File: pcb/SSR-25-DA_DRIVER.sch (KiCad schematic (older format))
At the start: 3 parts, among them Q3 SS9013_J3

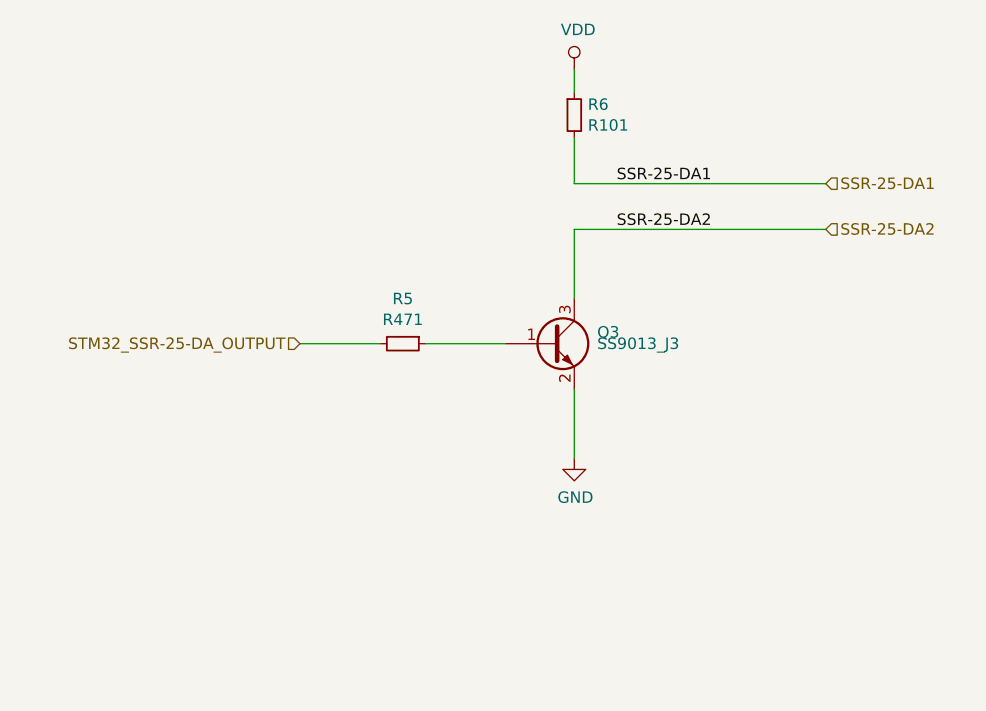
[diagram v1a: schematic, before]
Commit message: update,
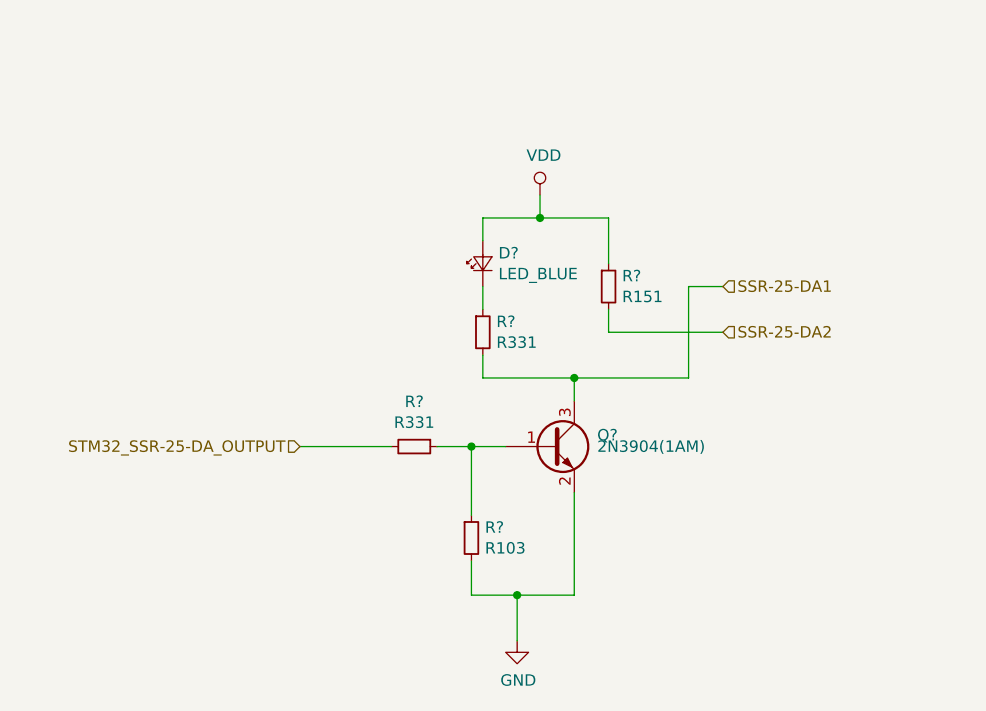
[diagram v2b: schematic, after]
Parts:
- removed Q3: SS9013_J3, Package_TO_SOT_SMD:SOT-23_Handsoldering, symbol taobao-transistor:SS9013_J3
- removed R5: R471, Resistor_SMD:R_0805_2012Metric_Pad1.15x1.40mm_HandSolder, symbol taobao-r:R471
- removed R6: R101, Resistor_SMD:R_0805_2012Metric_Pad1.15x1.40mm_HandSolder, symbol taobao-r:R101
- added D?: LED_BLUE, LED_SMD:LED_0805_2012Metric_Pad1.15x1.40mm_HandSolder, symbol taobao-components:LED_RED
- added Q?: 2N3904(1AM), Package_TO_SOT_SMD:SOT-23_Handsoldering, symbol taobao-transistor:2N3904(1AM)
- added R? (x2): R331, Resistor_SMD:R_0805_2012Metric_Pad1.15x1.40mm_HandSolder, symbol taobao-r:R331
- added R?: R103, Resistor_SMD:R_0805_2012Metric_Pad1.15x1.40mm_HandSolder, symbol taobao-r:R103
- added R?: R151, Resistor_SMD:R_0805_2012Metric_Pad1.15x1.40mm_HandSolder, symbol taobao-r:R151
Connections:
- net GND: now also Q?.2 (E), R?.2
- net SSR-25-DA1: now also Q?.3 (C), R?.2
- net SSR-25-DA2: now also R?.2
- net STM32_SSR-25-DA_OUTPUT: now also R?.2
- net VDD: now also D?.2 (A), R?.1
- new net: Q?.1 (B), R?.1, R?.1
- new net: D?.1 (K), R?.1
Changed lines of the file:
@@
 Comment4 ""
 $EndDescr
+Text HLabel 5050 3550 0    50   Input ~ 0
+STM32_SSR-25-DA_OUTPUT
 $Comp
-L power:VDD #PWR013
-U 1 1 5BCB697F
-P 6250 1900
-F 0 "#PWR013" H 6250 1750 50  0001 C CNN
-F 1 "VDD" H 6267 2073 50  0000 C CNN
-F 2 "" H 6250 1900 50  0001 C CNN
-F 3 "" H 6250 1900 50  0001 C CNN
-	1    6250 1900
-	1    0    0    -1
+L taobao-r:R331 R?
+U 1 1 5BDCB66A
+P 5550 3550
+AR Path="/5BCB4A39/5BDCB66A" Ref="R?"  Part="1"
+AR Path="/5BE41138/5BDCB66A" Ref="R?"  Part="1"
+AR Path="/5BCB679F/5BDCB66A" Ref="R?"  Part="1"
+F 0 "R?" V 5354 3550 50  0000 C CNN
+F 1 "R331" V 5445 3550 50  0000 C CNN
+F 2 "Resistor_SMD:R_0805_2012Metric_Pad1.15x1.40mm_HandSolder" H 5550 3550 50  0001 C CNN
+F 3 "~" H 5550 3550 50  0001 C CNN
+	1    5550 3550
+	0    1    1    0
 $EndComp
 $Comp
-L taobao-r:R101 R6
-U 1 1 5BCB69F8
-P 6250 2100
-F 0 "R6" H 6309 2146 50  0000 L CNN
-F 1 "R101" H 6309 2055 50  0000 L CNN
-F 2 "Resistor_SMD:R_0805_2012Metric_Pad1.15x1.40mm_HandSolder" H 6250 2100 50  0001 C CNN
-F 3 "~" H 6250 2100 50  0001 C CNN
-	1    6250 2100
-	1    0    0    -1
-$EndComp
-$Comp
-L taobao-r:R471 R5
-U 1 1 5BCB6A7C
-P 5500 3100
-F 0 "R5" V 5304 3100 50  0000 C CNN
-F 1 "R471" V 5395 3100 50  0000 C CNN
-F 2 "Resistor_SMD:R_0805_2012Metric_Pad1.15x1.40mm_HandSolder" H 5500 3100 50  0001 C CNN
-F 3 "~" H 5500 3100 50  0001 C CNN
-	1    5500 3100
-	0    1    1    0
-$EndComp
-Text Label 6850 2400 2    50   ~ 0
-SSR-25-DA1
-Text Label 6850 2600 2    50   ~ 0
-SSR-25-DA2
-Text HLabel 5050 3100 0    50   Input ~ 0
-STM32_SSR-25-DA_OUTPUT
-Wire Wire Line
-	5050 3100 5400 3100
-$Comp
-L power:GND #PWR014
-U 1 1 5BCB6BDC
-P 6250 3600
-F 0 "#PWR014" H 6250 3350 50  0001 C CNN
-F 1 "GND" H 6255 3427 50  0000 C CNN
-F 2 "" H 6250 3600 50  0001 C CNN
-F 3 "" H 6250 3600 50  0001 C CNN
-	1    6250 3600
+L taobao-r:R103 R?
+U 1 1 5BDCB672
+P 5800 3950
+AR Path="/5BCB4A39/5BDCB672" Ref="R?"  Part="1"
+AR Path="/5BE41138/5BDCB672" Ref="R?"  Part="1"
+AR Path="/5BCB679F/5BDCB672" Ref="R?"  Part="1"
+F 0 "R?" H 5859 3996 50  0000 L CNN
+F 1 "R103" H 5859 3905 50  0000 L CNN
+F 2 "Resistor_SMD:R_0805_2012Metric_Pad1.15x1.40mm_HandSolder" H 5800 3950 50  0001 C CNN
+F 3 "~" H 5800 3950 50  0001 C CNN
+	1    5800 3950
 	1    0    0    -1
 $EndComp
 Wire Wire Line
-	6250 3300 6250 3600
+	5050 3550 5450 3550
 Wire Wire Line
-	5600 3100 5950 3100
+	5650 3550 5800 3550
 Wire Wire Line
-	6250 2200 6250 2400
+	5800 3550 5800 3850
 Wire Wire Line
-	6250 1900 6250 2000
+	5950 3550 5800 3550
+Connection ~ 5800 3550
 Wire Wire Line
-	6250 2600 6250 2900
-Text HLabel 7350 2400 2    50   Input ~ 0
-SSR-25-DA1
-Text HLabel 7350 2600 2    50   Input ~ 0
-SSR-25-DA2
+	5800 4050 5800 4200
 Wire Wire Line
-	6250 2400 7350 2400
+	5800 4200 6000 4200
 Wire Wire Line
-	6250 2600 7350 2600
+	6250 4200 6250 3750
 $Comp
-L taobao-transistor:SS9013_J3 Q3
-U 1 1 5BCBD15E
-P 6150 3100
-AR Path="/5BCBD15E" Ref="Q3"  Part="1"
-AR Path="/5BCB679F/5BCBD15E" Ref="Q3"  Part="1"
-F 0 "Q3" H 6350 3150 50  0000 L CNN
-F 1 "SS9013_J3" H 6350 3100 50  0000 L CNN
-F 2 "Package_TO_SOT_SMD:SOT-23_Handsoldering" H 6350 3025 50  0001 L CIN
-F 3 "https://www.fairchildsemi.com/datasheets/2N/2N3904.pdf" H 6150 3100 50  0001 L CNN
-	1    6150 3100
+L power:GND #PWR?
+U 1 1 5BDCB681
+P 6000 4400
+AR Path="/5BCB4A39/5BDCB681" Ref="#PWR?"  Part="1"
+AR Path="/5BE41138/5BDCB681" Ref="#PWR?"  Part="1"
+F 0 "#PWR?" H 6000 4150 50  0001 C CNN
+F 1 "GND" H 6005 4227 50  0000 C CNN
+F 2 "" H 6000 4400 50  0001 C CNN
+F 3 "" H 6000 4400 50  0001 C CNN
+	1    6000 4400
 	1    0    0    -1
 $EndComp
+Wire Wire Line
+	6000 4400 6000 4200
+Connection ~ 6000 4200
+Wire Wire Line
+	6000 4200 6250 4200
+$Comp
+L taobao-components:LED_RED D?
+U 1 1 5BDCB68A
+P 5850 2750
+AR Path="/5BCB4A39/5BDCB68A" Ref="D?"  Part="1"
+AR Path="/5BE41138/5BDCB68A" Ref="D?"  Part="1"
+AR Path="/5BCB679F/5BDCB68A" Ref="D?"  Part="1"
+F 0 "D?" V 5896 2682 50  0000 R CNN
+F 1 "LED_BLUE" V 5805 2682 50  0000 R CNN
+F 2 "LED_SMD:LED_0805_2012Metric_Pad1.15x1.40mm_HandSolder" V 5850 2750 50  0001 C CNN
+F 3 "~" V 5850 2750 50  0001 C CNN
+	1    5850 2750
+	0    -1   -1   0
+$EndComp
+$Comp
+L taobao-r:R331 R?
+U 1 1 5BDCB691
+P 5850 3050
+AR Path="/5BCB4A39/5BDCB691" Ref="R?"  Part="1"
+AR Path="/5BE41138/5BDCB691" Ref="R?"  Part="1"
+AR Path="/5BCB679F/5BDCB691" Ref="R?"  Part="1"
+F 0 "R?" H 5909 3096 50  0000 L CNN
+F 1 "R331" H 5909 3005 50  0000 L CNN
+F 2 "Resistor_SMD:R_0805_2012Metric_Pad1.15x1.40mm_HandSolder" H 5850 3050 50  0001 C CNN
+F 3 "~" H 5850 3050 50  0001 C CNN
+	1    5850 3050
+	1    0    0    -1
+$EndComp
+Wire Wire Line
+	5850 3150 5850 3250
+Wire Wire Line
+	5850 3250 6250 3250
+Wire Wire Line
+	6250 3250 6250 3350
+Wire Wire Line
+	5850 2550 5850 2650
+Wire Wire Line
+	5850 2850 5850 2950
+$Comp
+L taobao-r:R151 R?
+U 1 1 5BDCB69D
+P 6400 2850
+AR Path="/5BCB4A39/5BDCB69D" Ref="R?"  Part="1"
+AR Path="/5BE41138/5BDCB69D" Ref="R?"  Part="1"
+F 0 "R?" H 6459 2896 50  0000 L CNN
+F 1 "R151" H 6459 2805 50  0000 L CNN
+F 2 "Resistor_SMD:R_0805_2012Metric_Pad1.15x1.40mm_HandSolder" H 6400 2850 50  0001 C CNN
+F 3 "~" H 6400 2850 50  0001 C CNN
+	1    6400 2850
+	1    0    0    -1
+$EndComp
+Wire Wire Line
+	6400 2550 6400 2750
+Wire Wire Line
+	6400 2950 6400 3050
+Wire Wire Line
+	6400 3050 6900 3050
+Wire Wire Line
+	6250 3250 6750 3250
+Wire Wire Line
+	6750 3250 6750 2850
+Wire Wire Line
+	6750 2850 6900 2850
+Connection ~ 6250 3250
+$Comp
+L power:VDD #PWR?
+U 1 1 5BDCB6B8
+P 6100 2450
+AR Path="/5BCB4A39/5BDCB6B8" Ref="#PWR?"  Part="1"
+AR Path="/5BE41138/5BDCB6B8" Ref="#PWR?"  Part="1"
+F 0 "#PWR?" H 6100 2300 50  0001 C CNN
+F 1 "VDD" H 6117 2623 50  0000 C CNN
+F 2 "" H 6100 2450 50  0001 C CNN
+F 3 "" H 6100 2450 50  0001 C CNN
+	1    6100 2450
+	1    0    0    -1
+$EndComp
+Wire Wire Line
+	6100 2450 6100 2550
+Wire Wire Line
+	6100 2550 5850 2550
+Wire Wire Line
+	6100 2550 6400 2550
+Connection ~ 6100 2550
+$Comp
+L taobao-transistor:2N3904(1AM) Q?
+U 1 1 5BDCB6C2
+P 6150 3550
+AR Path="/5BDCB6C2" Ref="Q?"  Part="1"
+AR Path="/5BCB4A39/5BDCB6C2" Ref="Q?"  Part="1"
+AR Path="/5BE41138/5BDCB6C2" Ref="Q?"  Part="1"
+AR Path="/5BCB679F/5BDCB6C2" Ref="Q?"  Part="1"
+F 0 "Q?" H 6350 3600 50  0000 L CNN
+F 1 "2N3904(1AM)" H 6350 3550 50  0000 L CNN
+F 2 "Package_TO_SOT_SMD:SOT-23_Handsoldering" H 6350 3475 50  0001 L CIN
+F 3 "" H 6150 3550 50  0001 L CNN
+	1    6150 3550
+	1    0    0    -1
+$EndComp
+Text HLabel 6900 2850 2    50   Input ~ 0
+SSR-25-DA1
+Text HLabel 6900 3050 2    50   Input ~ 0
+SSR-25-DA2
 $EndSCHEMATC
